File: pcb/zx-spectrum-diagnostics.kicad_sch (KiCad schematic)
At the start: 19 parts, among them J101 Conn_01x04, J102 Conn_01x03_Male, J103 Conn_01x03_Male, Q101 PMBT2222A, SW101 SW_SPST, SW102 SW_SPST, U101 Pico, U102 Pico

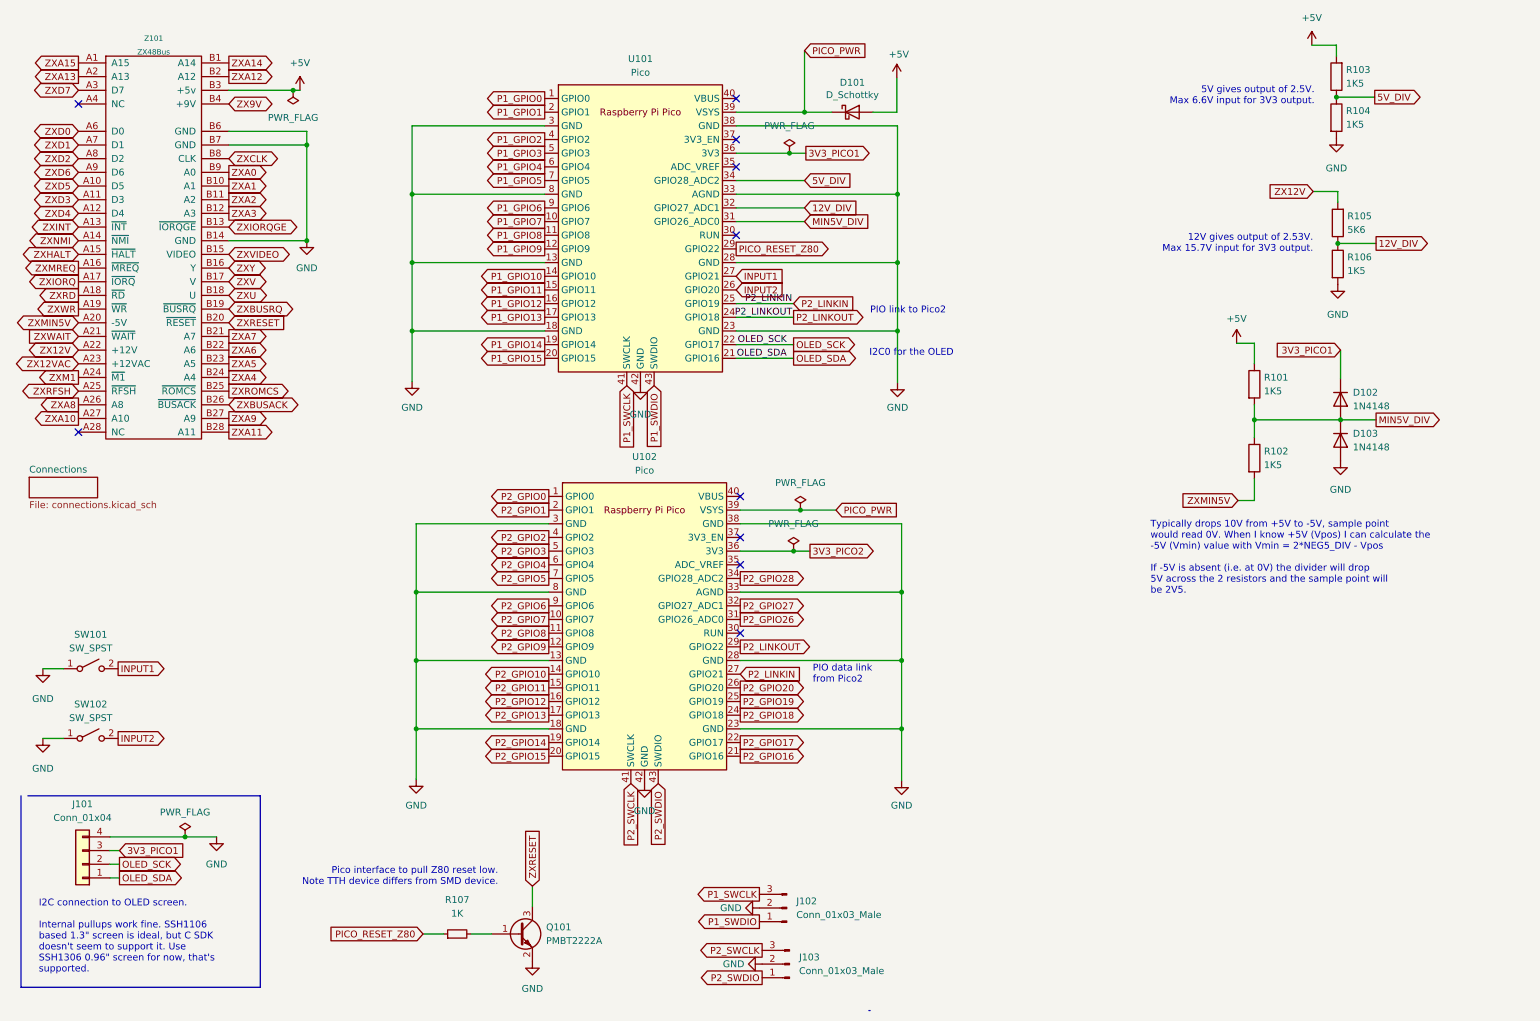
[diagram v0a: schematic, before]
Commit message: schematic reworked, it's time to relayout the board. checkpoint here
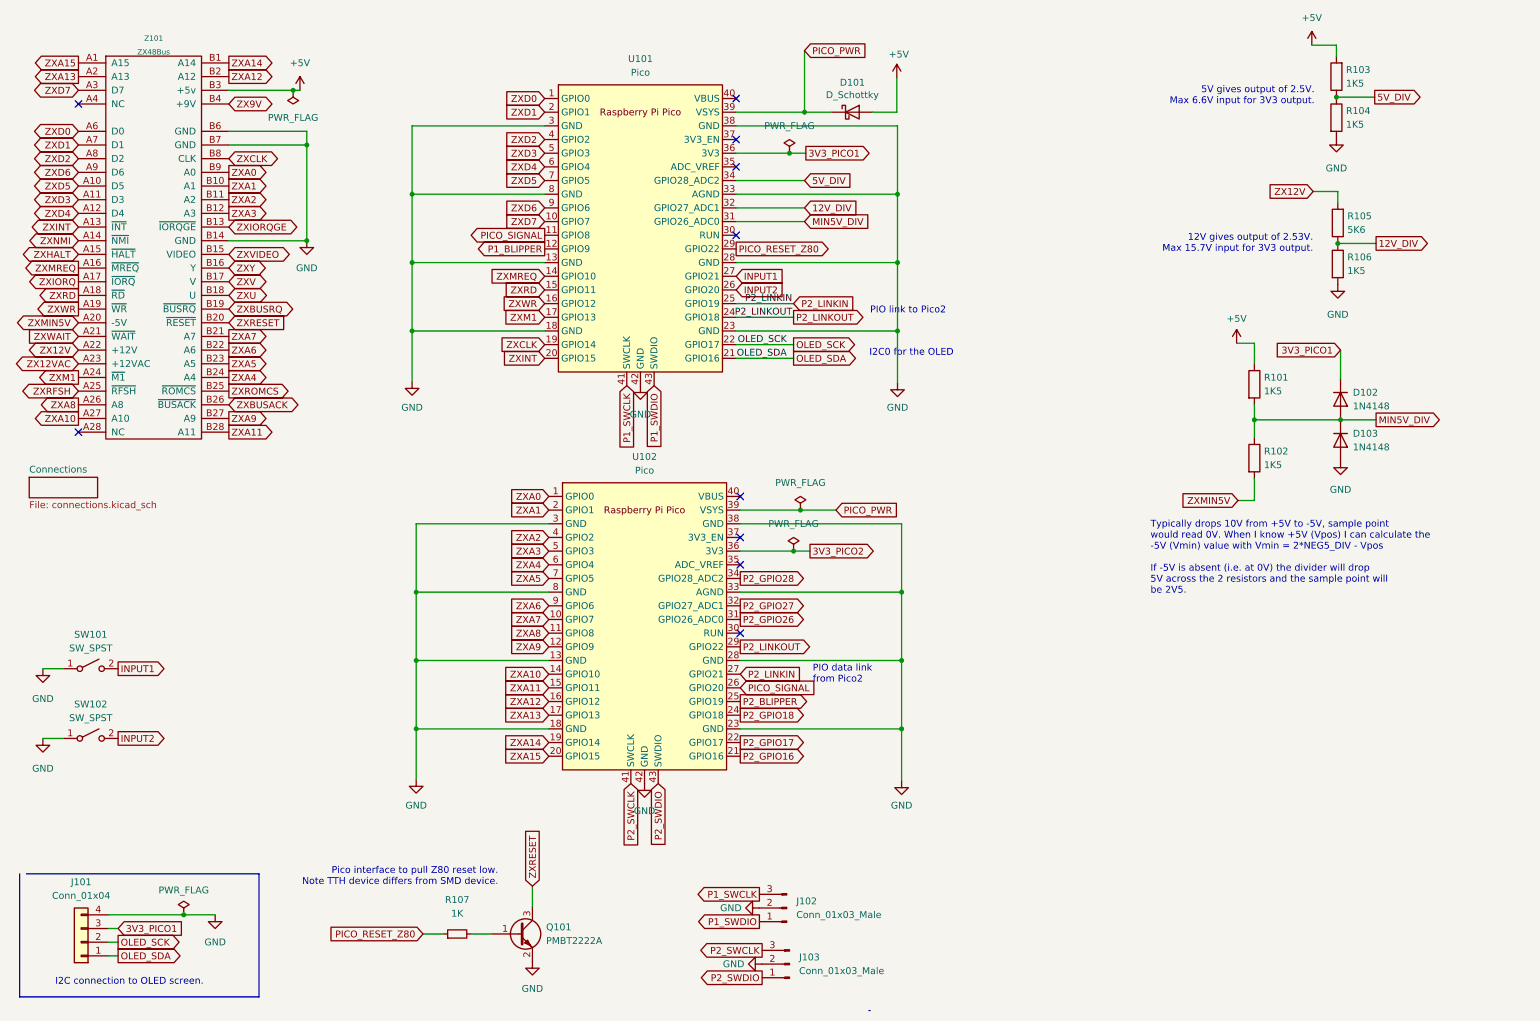
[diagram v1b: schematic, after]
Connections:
- net P1_GPIO0 is gone; now on net ZXD0: U101.1 (GPIO0)
- net P1_GPIO1 is gone; now on net ZXD1: U101.2 (GPIO1)
- net P1_GPIO10 is gone; now on net ZXMREQ: U101.14 (GPIO10)
- net P1_GPIO11 is gone; now on net ZXRD: U101.15 (GPIO11)
- net P1_GPIO12 is gone; now on net ZXWR: U101.16 (GPIO12)
- net P1_GPIO13 is gone; now on net ZXM1: U101.17 (GPIO13)
- net P1_GPIO14 is gone; now on net ZXCLK: U101.19 (GPIO14)
- net P1_GPIO15 is gone; now on net ZXINT: U101.20 (GPIO15)
- net P1_GPIO2 is gone; now on net ZXD2: U101.4 (GPIO2)
- net P1_GPIO3 is gone; now on net ZXD3: U101.5 (GPIO3)
- net P1_GPIO4 is gone; now on net ZXD4: U101.6 (GPIO4)
- net P1_GPIO5 is gone; now on net ZXD5: U101.7 (GPIO5)
- net P1_GPIO6 is gone; now on net ZXD6: U101.9 (GPIO6)
- net P1_GPIO7 is gone; now on net ZXD7: U101.10 (GPIO7)
- net P2_GPIO0 is gone; now on net ZXA0: U102.1 (GPIO0)
- net P2_GPIO1 is gone; now on net ZXA1: U102.2 (GPIO1)
- net P2_GPIO10 is gone; now on net ZXA10: U102.14 (GPIO10)
- net P2_GPIO11 is gone; now on net ZXA11: U102.15 (GPIO11)
- net P2_GPIO12 is gone; now on net ZXA12: U102.16 (GPIO12)
- net P2_GPIO13 is gone; now on net ZXA13: U102.17 (GPIO13)
- net P2_GPIO14 is gone; now on net ZXA14: U102.19 (GPIO14)
- net P2_GPIO15 is gone; now on net ZXA15: U102.20 (GPIO15)
- net P2_GPIO2 is gone; now on net ZXA2: U102.4 (GPIO2)
- net P2_GPIO20 is gone; now on net PICO_SIGNAL: U102.26 (GPIO20)
- net P2_GPIO3 is gone; now on net ZXA3: U102.5 (GPIO3)
- net P2_GPIO4 is gone; now on net ZXA4: U102.6 (GPIO4)
- net P2_GPIO5 is gone; now on net ZXA5: U102.7 (GPIO5)
- net P2_GPIO6 is gone; now on net ZXA6: U102.9 (GPIO6)
- net P2_GPIO7 is gone; now on net ZXA7: U102.10 (GPIO7)
- net P2_GPIO8 is gone; now on net ZXA8: U102.11 (GPIO8)
- net P2_GPIO9 is gone; now on net ZXA9: U102.12 (GPIO9)
- net P1_GPIO8 renamed PICO_SIGNAL
- net P1_GPIO9 renamed P1_BLIPPER
- net P2_GPIO19 renamed P2_BLIPPER
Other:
- note added: "I2C connection to OLED screen."
- note removed: "I2C connection to OLED screen. Internal pullups work fine. SSH1106 based 1.3" screen is ideal, but C SDK doesn't seem to support it. Use SSH1306 0.96" screen for now, that's supported."
- moved on the sheet: J101
